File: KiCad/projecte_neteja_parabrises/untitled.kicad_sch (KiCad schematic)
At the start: 16 parts, among them J2 DE9_Pins, J3 DE9_Pins, SW1 CALEFACTOR, SW2 BOMBAS, SW3 SW_SP5T_NR01105, U8 TJA1049TK-3, U9 MAX232

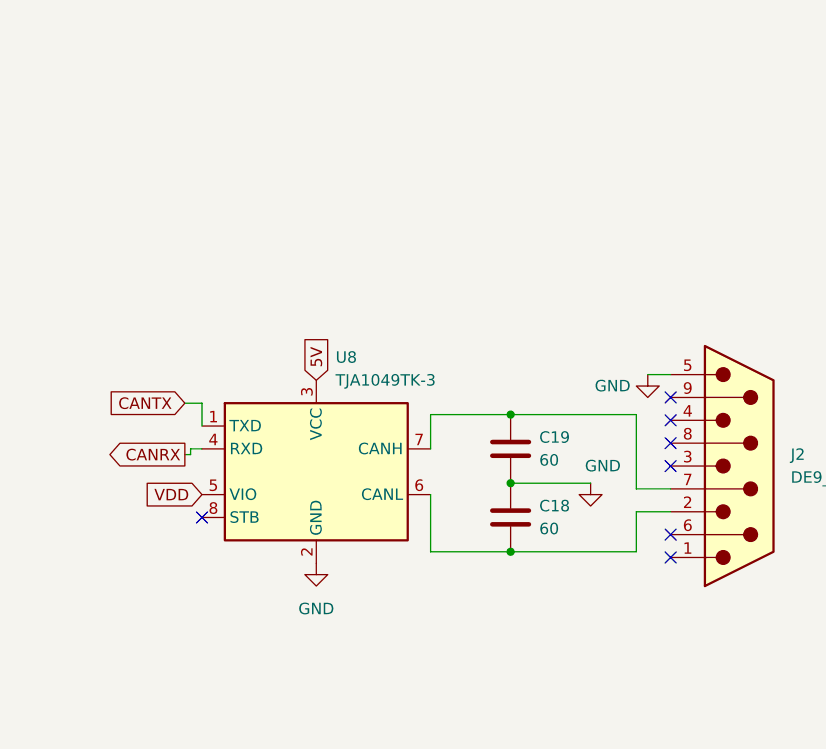
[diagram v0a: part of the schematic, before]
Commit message: detector lluvia
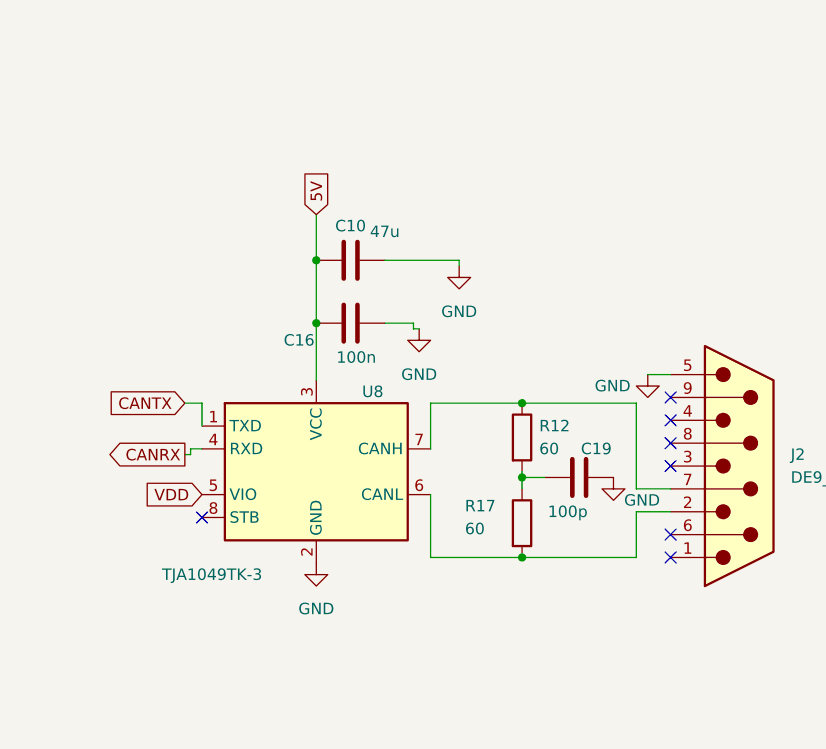
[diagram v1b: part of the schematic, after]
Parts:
- removed C18: 60, Capacitor_SMD:C_0805_2012Metric, symbol Device:C
- added C10: 47u, symbol Device:C
- added C16: 100n, symbol Device:C
- added R12, R17: 60, symbol Device:R
- C19: value 60 -> 100p
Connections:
- net 5V: now also C10.1, C16.1
- net GND: now also C10.2, C16.2
- net at J2.2, U8.6 (CANL): now also R17.2
- net at J2.7, U8.7 (CANH): now also R12.1; no longer C19.1
- new net: C19.1, R12.2, R17.1
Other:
- moved on the sheet: C19

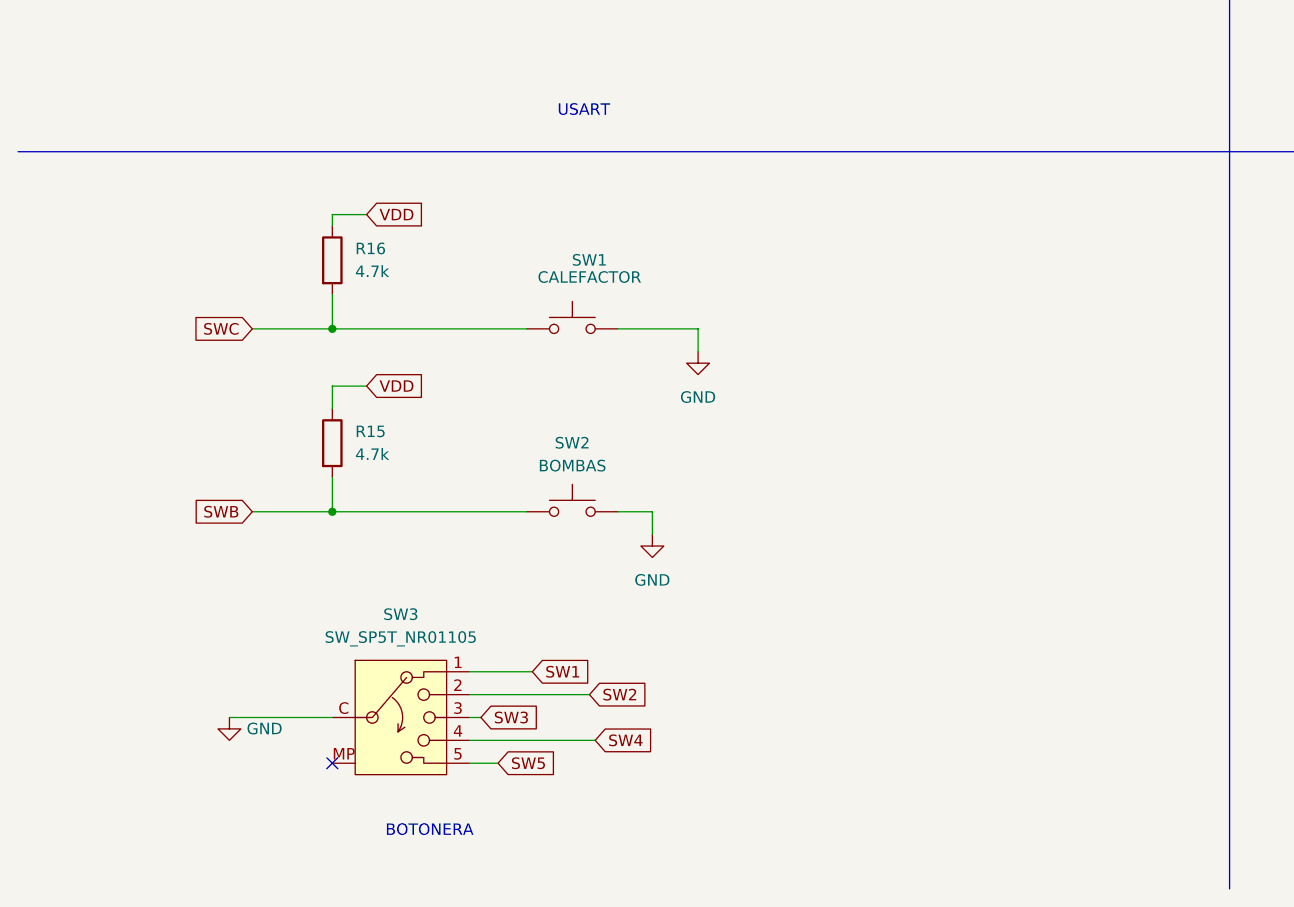
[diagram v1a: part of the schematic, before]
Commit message: Botonera
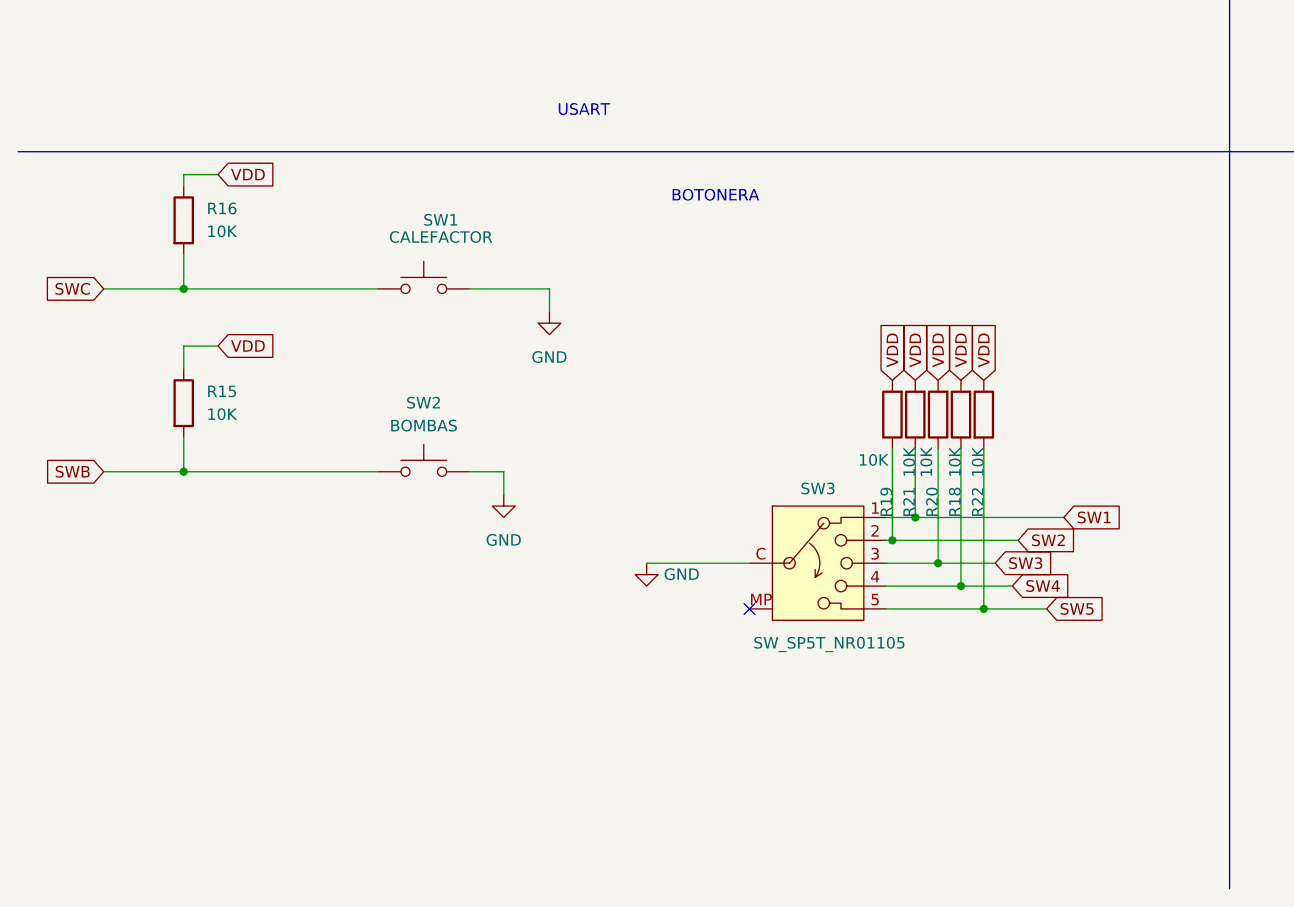
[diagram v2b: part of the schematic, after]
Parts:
- added R18, R19, R20, R21, R22: 10K, Resistor_SMD:R_0201_0603Metric_Pad0.64x0.40mm_HandSolder, symbol Device:R
- C10: footprint (none) -> Capacitor_SMD:C_0805_2012Metric_Pad1.18x1.45mm_HandSolder
- C16: footprint (none) -> Capacitor_SMD:C_0805_2012Metric
- R12, R17: footprint (none) -> Resistor_SMD:R_0201_0603Metric_Pad0.64x0.40mm_HandSolder
- R15, R16: value 4.7k -> 10K
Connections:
- net SW1: now also R21.1
- net SW2: now also R19.1
- net SW3: now also R20.1
- net SW4: now also R18.1
- net SW5: now also R22.2
- net VDD: now also R18.2, R19.2, R20.2, R21.2, R22.1
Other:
- moved on the sheet: R15, R16, SW1, SW2, SW3

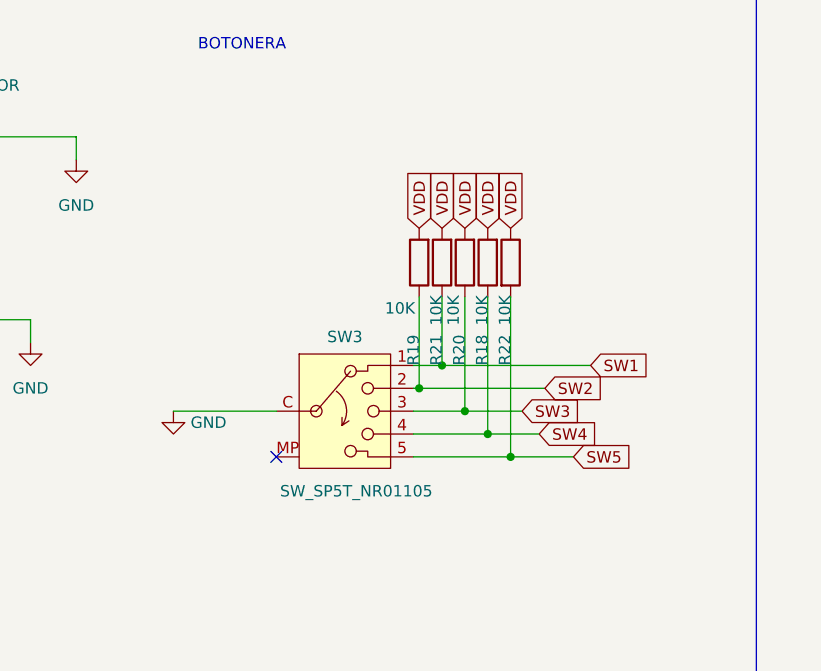
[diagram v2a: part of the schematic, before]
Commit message: POTENCIA GND
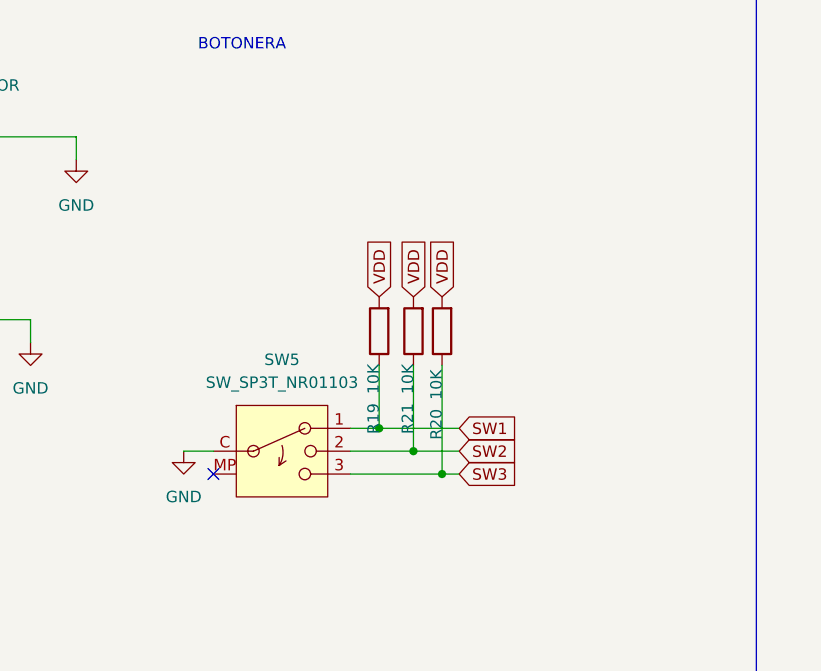
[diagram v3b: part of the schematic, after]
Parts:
- removed R18, R22: 10K, Resistor_SMD:R_0201_0603Metric_Pad0.64x0.40mm_HandSolder, symbol Device:R
- removed SW3: SW_SP5T_NR01105, Button_Switch_THT:SW_NKK_NR01, symbol Switch:SW_SP5T_NR01105
- added SW5: SW_SP3T_NR01103, Button_Switch_THT:SW_NKK_NR01, symbol Switch:SW_SP3T_NR01103
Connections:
- net GND: now also SW5.C (Common)
- net SW1: now also R19.1, SW5.1; no longer R21.1
- net SW2: now also R21.1, SW5.2; no longer R19.1
- net SW3: now also SW5.3
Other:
- moved on the sheet: R19, R20, R21

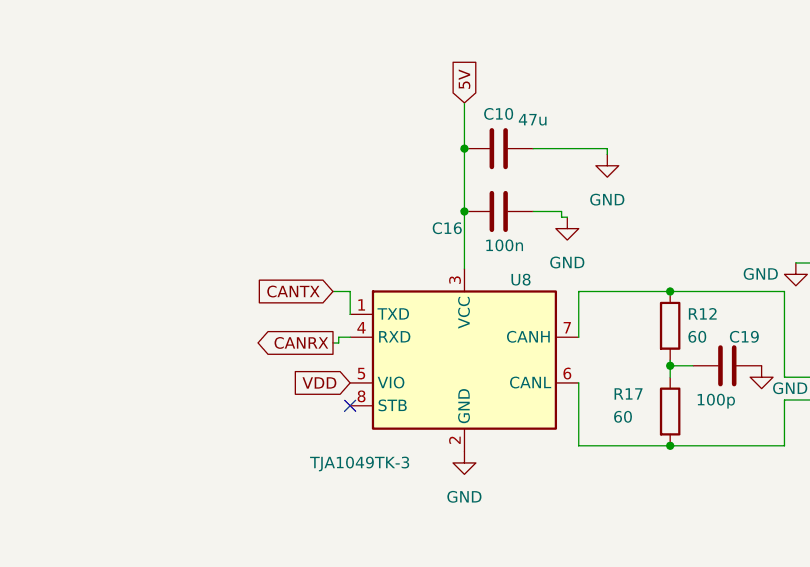
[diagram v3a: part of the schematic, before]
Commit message: huella ferrita
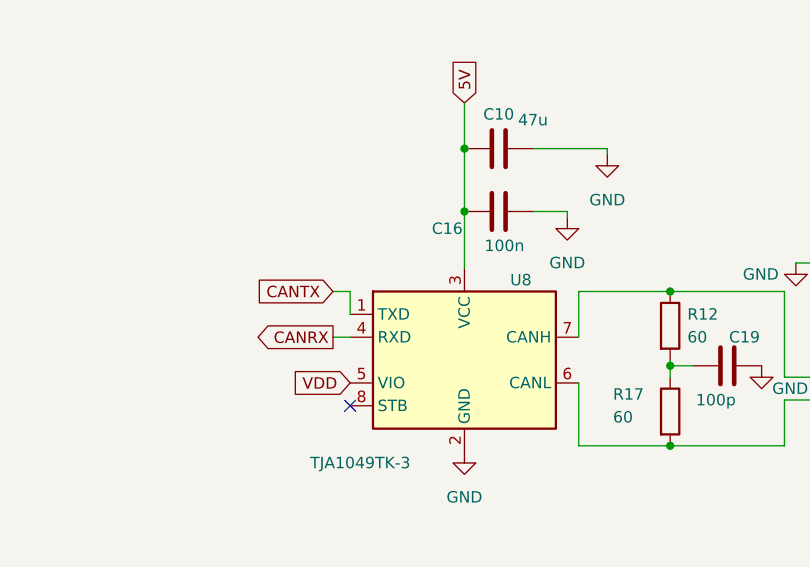
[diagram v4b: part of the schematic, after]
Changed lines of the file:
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@@
 	(wire
 		(pts
-			(xy 193.04 65.405) (xy 193.675 65.405)
+			(xy 193.04 64.77) (xy 194.945 64.77)
 		)
 		(stroke
@@
 	(wire
 		(pts
-			(xy 219.075 51.435) (xy 218.44 51.435)
-		)
-		(stroke
-			(width 0)
-			(type default)
-		)
-	)
-	(wire
-		(pts
 			(xy 230.505 76.835) (xy 243.205 76.835)
 		)
@@
 	(wire
 		(pts
-			(xy 193.675 64.77) (xy 193.675 65.405)
-		)
-		(stroke
-			(width 0)
-			(type default)
-		)
-	)
-	(wire
-		(pts
 			(xy 30.48 137.795) (xy 34.29 137.795)
 		)
@@
 	(wire
 		(pts
-			(xy 218.44 51.435) (xy 218.44 50.8)
-		)
-		(stroke
-			(width 0)
-			(type default)
-		)
-	)
-	(wire
-		(pts
 			(xy 71.12 131.445) (xy 71.12 133.985)
 		)
@@
 	(wire
 		(pts
-			(xy 218.44 50.8) (xy 215.265 50.8)
+			(xy 215.265 50.8) (xy 219.075 50.8)
 		)
 		(stroke
@@
 	(wire
 		(pts
-			(xy 193.675 64.77) (xy 194.945 64.77)
-		)
-		(stroke
-			(width 0)
-			(type default)
-		)
-	)
-	(wire
-		(pts
 			(xy 84.455 64.77) (xy 84.455 76.2)
 		)
@@
 		(pts
 			(xy 243.205 71.755) (xy 247.015 71.755)
+		)
+		(stroke
+			(width 0)
+			(type default)
+		)
+	)
+	(wire
+		(pts
+			(xy 219.075 50.8) (xy 219.075 51.435)
 		)
 		(stroke
@@
 	(global_label "CANRX"
 		(shape output)
-		(at 193.04 65.405 180)
+		(at 193.04 64.77 180)
 		(fields_autoplaced yes)
 		(effects
@@
 		)
 		(property "Intersheetrefs" "${INTERSHEET_REFS}"
-			(at 183.8862 65.405 0)
+			(at 183.8862 64.77 0)
 			(effects
 				(font
